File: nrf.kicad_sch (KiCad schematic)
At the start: 41 parts, among them J1 USB_C_Receptacle_USB2.0_16P, Q1 lpo404, SW1 RESET, U1 nRF52840, U2 BQ25101YFPR, Y1 32.768kHz, Y2 32mHz

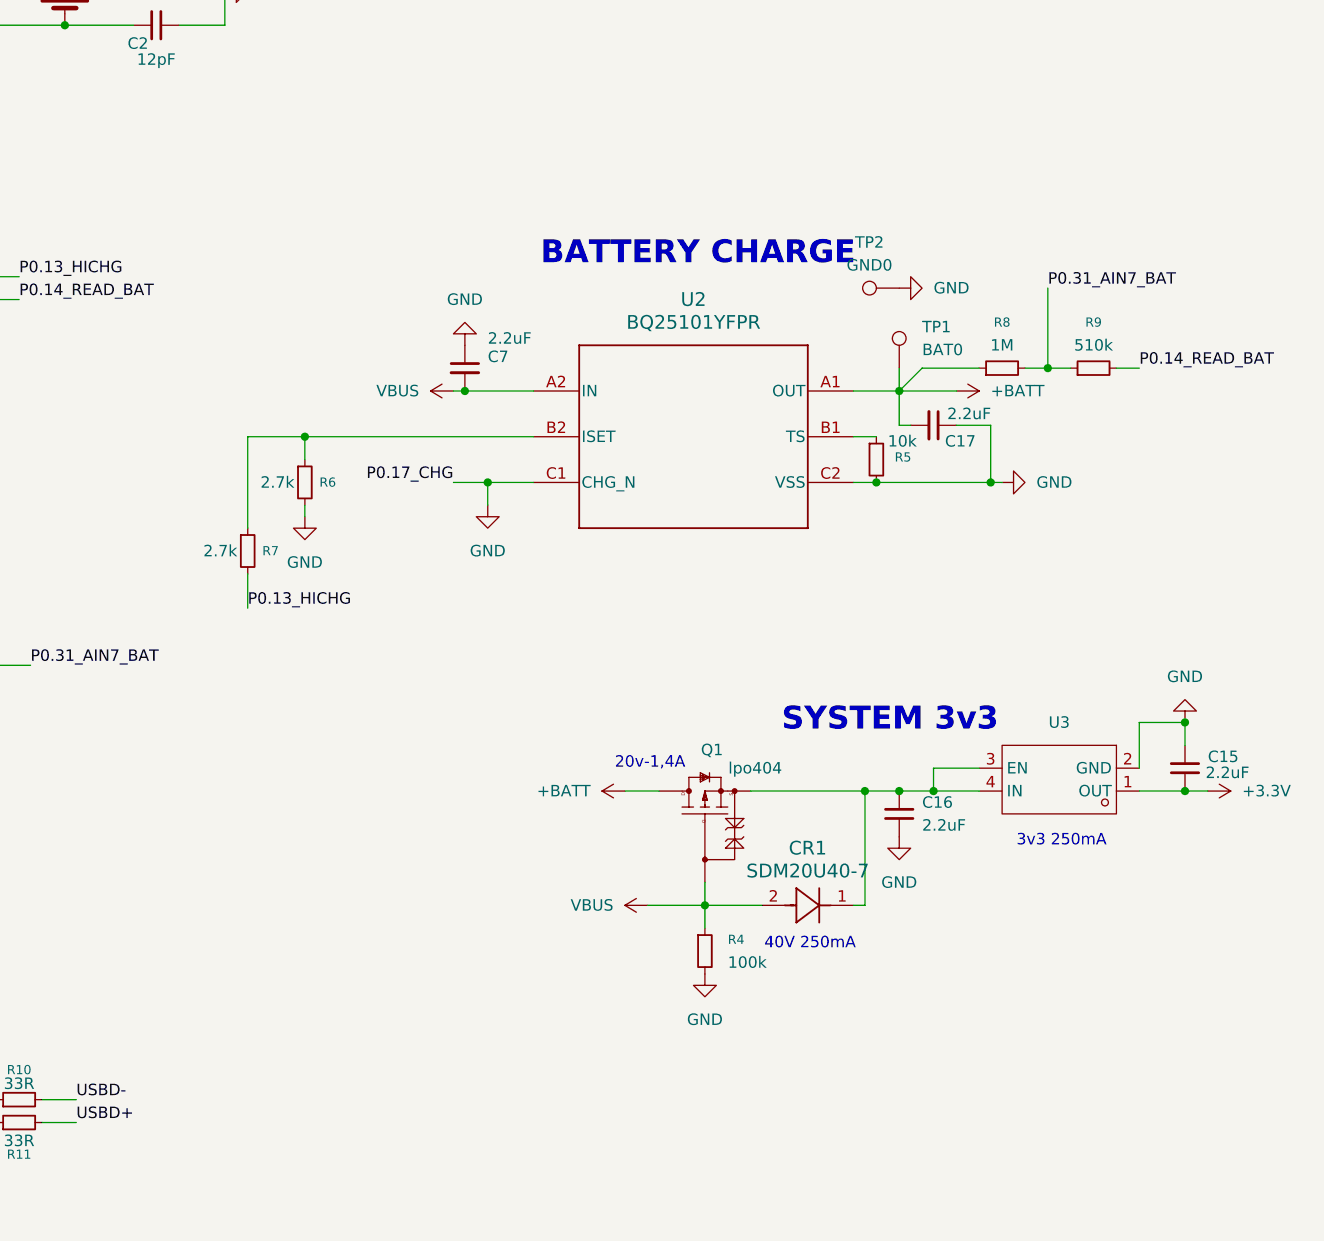
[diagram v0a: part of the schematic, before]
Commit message: Dodanie ledu
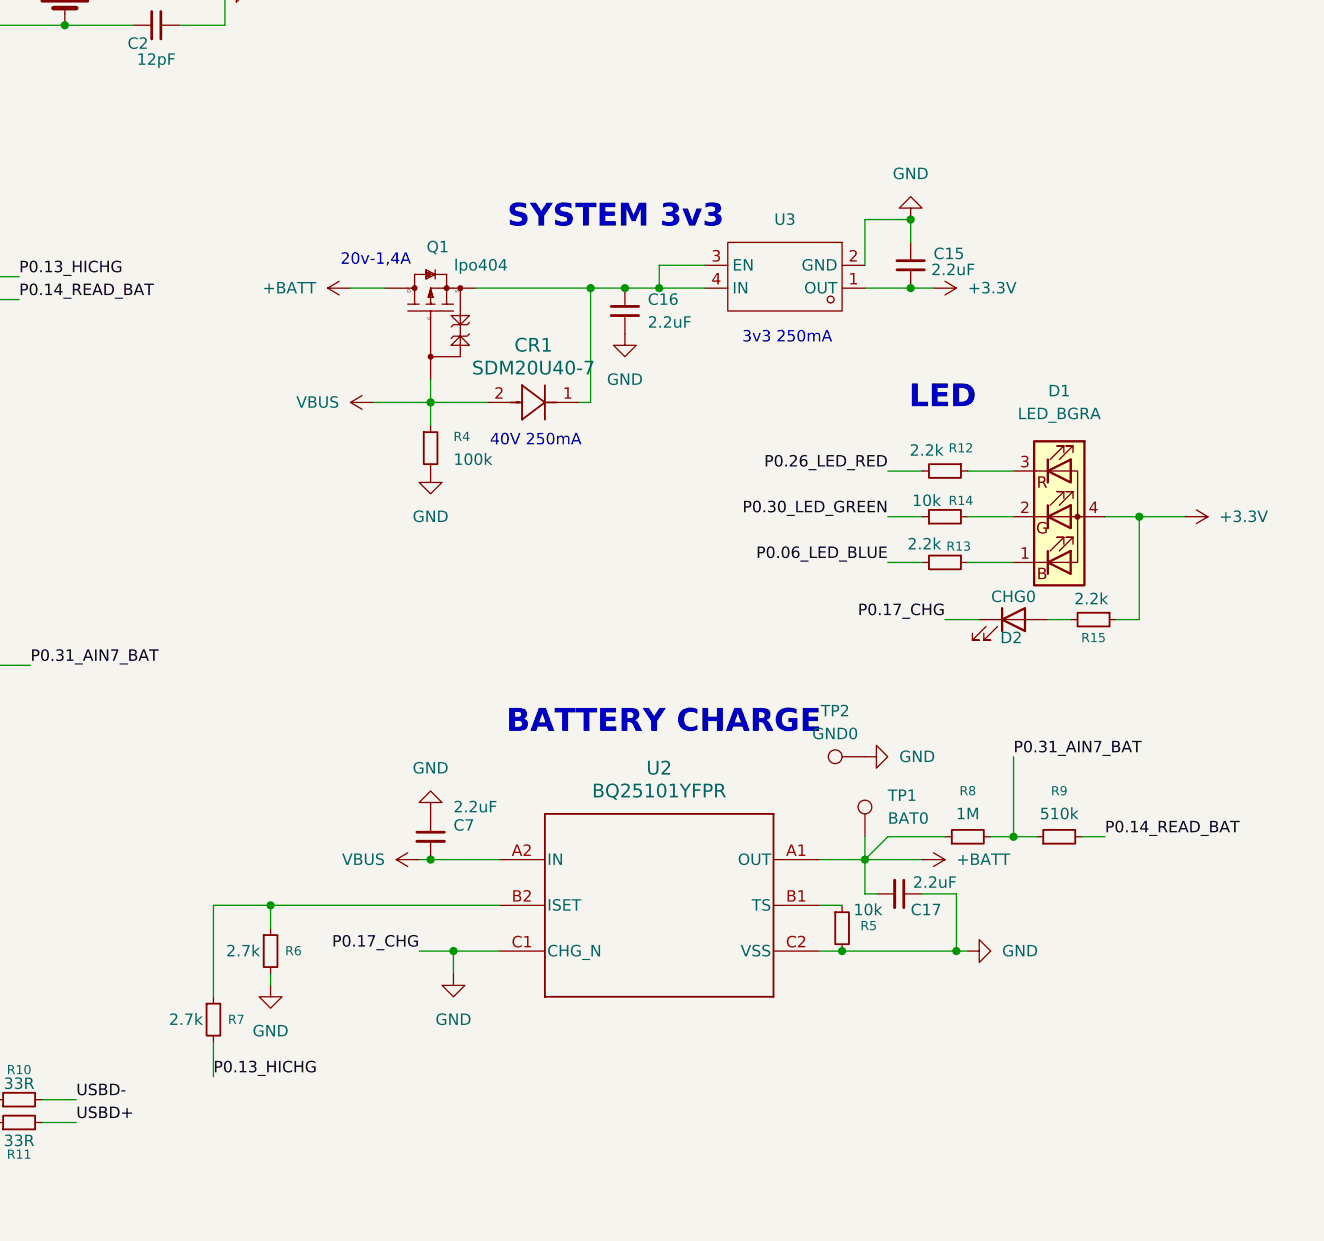
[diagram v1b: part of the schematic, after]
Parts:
- added D1: LED_BGRA, symbol Device:LED_BGRA
- added D2: CHG0, symbol Device:LED
- added R12, R13, R15: 2.2k, symbol Device:R_Small
- added R14: 10k, symbol Device:R_Small
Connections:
- net +3.3V: now also D1.4 (A), R15.1
- net GND: now also D2.1 (K)
- new net: D2.2 (A), R15.2
- new net: D1.1 (BK), R13.1
- new net: D1.2 (GK), R14.2
- new net: D1.3 (RK), R12.1
- new net P0.06_LED_BLUE: R13.2
- new net P0.26_LED_RED: R12.2
- new net P0.30_LED_GREEN: R14.1
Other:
- note added: "LED"
- moved on the sheet: C15, C16, C17, C7, CR1, Q1, R4, R5, R6, R7, R8, R9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
